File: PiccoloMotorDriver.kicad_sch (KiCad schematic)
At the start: 4 parts

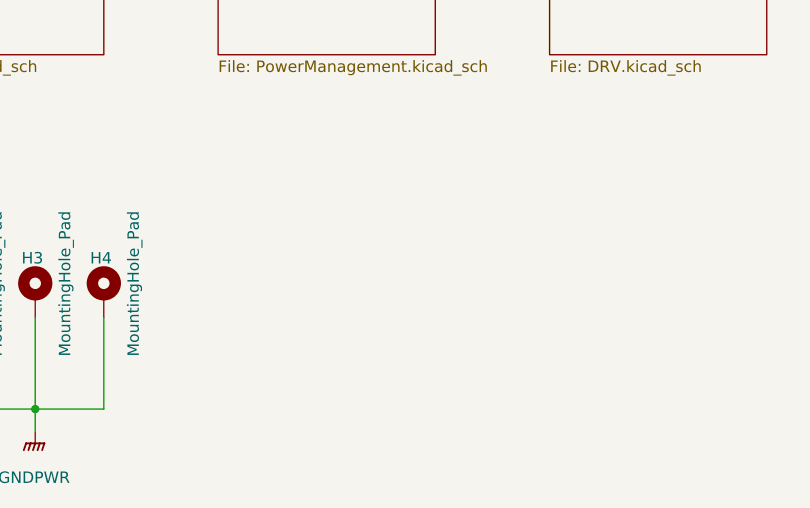
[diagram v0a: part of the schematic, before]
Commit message: more layout
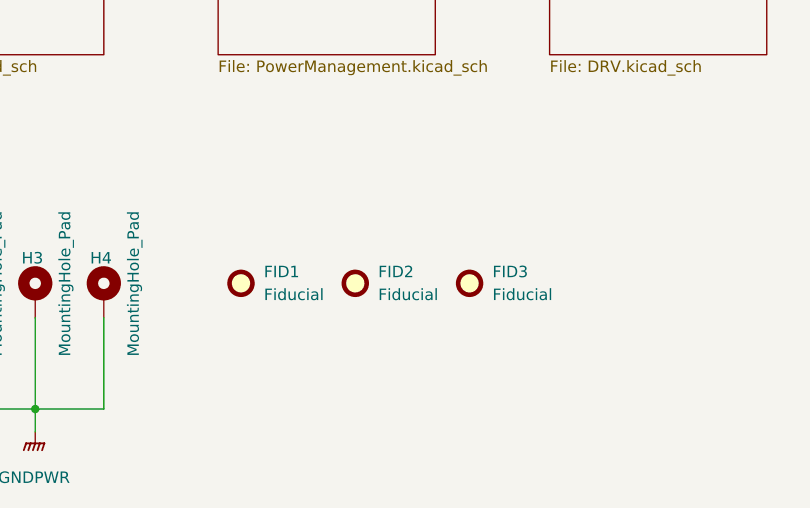
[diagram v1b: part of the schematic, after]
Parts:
- added FID1, FID2, FID3: Fiducial, Fiducial:Fiducial_0.5mm_Mask1mm, symbol Mechanical:Fiducial
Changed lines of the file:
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@@
+	)
+	(symbol
+		(lib_id "Mechanical:Fiducial")
+		(at 85.09 68.58 0)
+		(unit 1)
+		(exclude_from_sim no)
+		(in_bom no)
+		(on_board yes)
+		(dnp no)
+		(fields_autoplaced yes)
+		(property "Reference" "FID3"
+			(at 87.63 67.3099 0)
+			(effects
+				(font
+					(size 1.27 1.27)
+				)
+				(justify left)
+			)
+		)
+		(property "Value" "Fiducial"
+			(at 87.63 69.8499 0)
+			(effects
+				(font
+					(size 1.27 1.27)
+				)
+				(justify left)
+			)
+		)
+		(property "Footprint" "Fiducial:Fiducial_0.5mm_Mask1mm"
+			(at 85.09 68.58 0)
+			(effects
+				(font
+					(size 1.27 1.27)
+				)
+				(hide yes)
+			)
+		)
+		(property "Datasheet" "~"
+			(at 85.09 68.58 0)
+			(effects
+				(font
+					(size 1.27 1.27)
+				)
+				(hide yes)
+			)
+		)
+		(property "Description" "Fiducial Marker"
+			(at 85.09 68.58 0)
+			(effects
+				(font
+					(size 1.27 1.27)
+				)
+				(hide yes)
+			)
+		)
+		(instances
+			(project ""
+				(path "/cc8a13e7-b1a6-4cbd-adcd-4feb8b2e2369"
+					(reference "FID3")
+					(unit 1)
+				)
+			)
+		)
 	)
 	(symbol
@@
 	)
 	(symbol
+		(lib_id "Mechanical:Fiducial")
+		(at 72.39 68.58 0)
+		(unit 1)
+		(exclude_from_sim no)
+		(in_bom no)
+		(on_board yes)
+		(dnp no)
+		(fields_autoplaced yes)
+		(property "Reference" "FID2"
+			(at 74.93 67.3099 0)
+			(effects
+				(font
+					(size 1.27 1.27)
+				)
+				(justify left)
+			)
+		)
+		(property "Value" "Fiducial"
+			(at 74.93 69.8499 0)
+			(effects
+				(font
+					(size 1.27 1.27)
+				)
+				(justify left)
+			)
+		)
+		(property "Footprint" "Fiducial:Fiducial_0.5mm_Mask1mm"
+			(at 72.39 68.58 0)
+			(effects
+				(font
+					(size 1.27 1.27)
+				)
+				(hide yes)
+			)
+		)
+		(property "Datasheet" "~"
+			(at 72.39 68.58 0)
+			(effects
+				(font
+					(size 1.27 1.27)
+				)
+				(hide yes)
+			)
+		)
+		(property "Description" "Fiducial Marker"
+			(at 72.39 68.58 0)
+			(effects
+				(font
+					(size 1.27 1.27)
+				)
+				(hide yes)
+			)
+		)
+		(instances
+			(project ""
+				(path "/cc8a13e7-b1a6-4cbd-adcd-4feb8b2e2369"
+					(reference "FID2")
+					(unit 1)
+				)
+			)
+		)
+	)
+	(symbol
 		(lib_id "Mechanical:MountingHole_Pad")
 		(at 21.59 69.85 0)
@@
 					(unit 1)
 				)
+			)
+		)
+	)
+	(symbol
+		(lib_id "Mechanical:Fiducial")
+		(at 59.69 68.58 0)
+		(unit 1)
+		(exclude_from_sim no)
+		(in_bom no)
+		(on_board yes)
+		(dnp no)
+		(fields_autoplaced yes)
+		(property "Reference" "FID1"
+			(at 62.23 67.3099 0)
+			(effects
+				(font
+					(size 1.27 1.27)
+				)
+				(justify left)
+			)
+		)
+		(property "Value" "Fiducial"
+			(at 62.23 69.8499 0)
+			(effects
+				(font
+					(size 1.27 1.27)
+				)
+				(justify left)
+			)
+		)
+		(property "Footprint" "Fiducial:Fiducial_0.5mm_Mask1mm"
+			(at 59.69 68.58 0)
+			(effects
+				(font
+					(size 1.27 1.27)
+				)
+				(hide yes)
+			)
+		)
+		(property "Datasheet" "~"
+			(at 59.69 68.58 0)
+			(effects
+				(font
+					(size 1.27 1.27)
+				)
+				(hide yes)
+			)
+		)
+		(property "Description" "Fiducial Marker"
+			(at 59.69 68.58 0)
+			(effects
+				(font
+					(size 1.27 1.27)
+				)
+				(hide yes)
+			)
+		)
+		(instances
+			(project ""
+				(path "/cc8a13e7-b1a6-4cbd-adcd-4feb8b2e2369"
+					(reference "FID1")
+					(unit 1)
+				)
